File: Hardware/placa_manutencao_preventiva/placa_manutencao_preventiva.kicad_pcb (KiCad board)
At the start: 2 copper layers, 58.4 x 74.7 mm, 23 parts, among them J1 ENT_DIGITAL, J2 Power, J3 TESTE_TENSAO, J4 BAT_EXT, J5 BAT_HELTEC_CONN, J6 MPU6050, J7 BMP180, J8 Renewable energy, Q2 FQP30N06L, U1 Heltec_Wifi_LoRa_V1, U2 LM7805

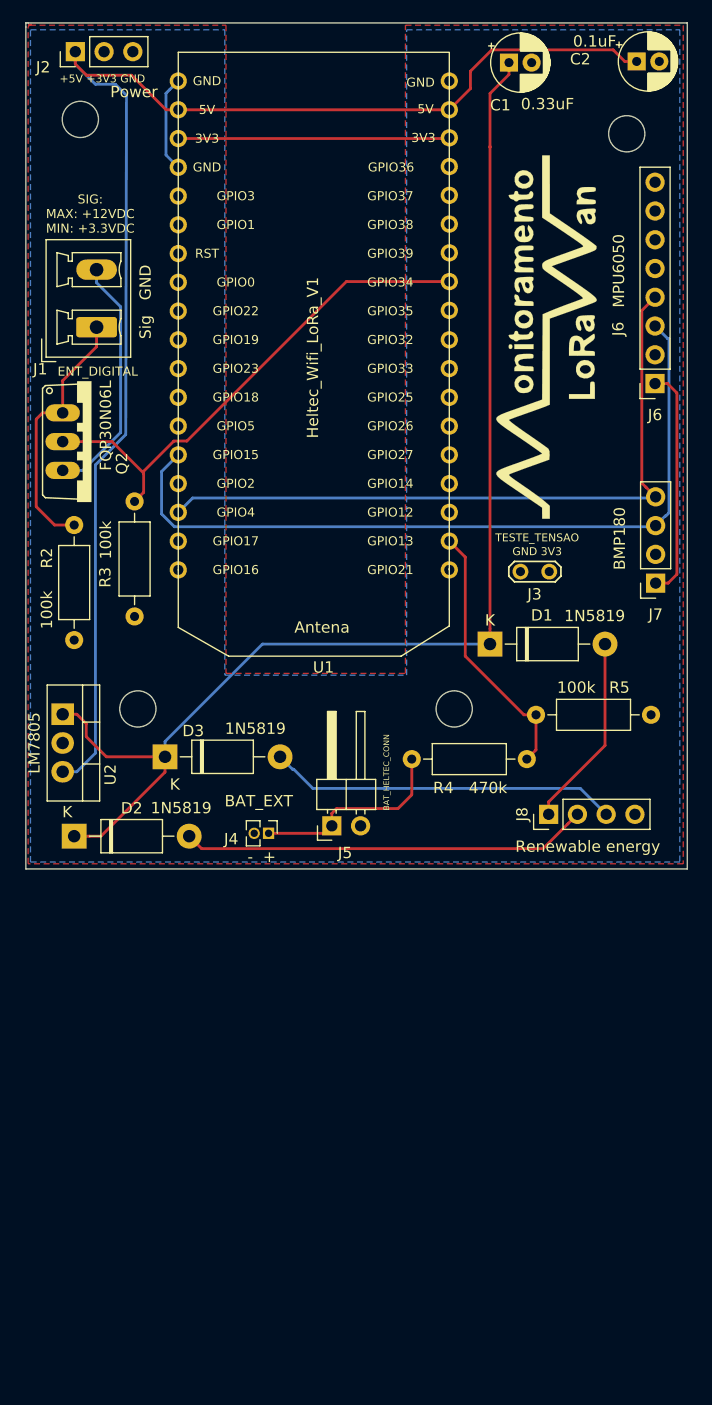
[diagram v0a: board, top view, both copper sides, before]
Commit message: Vers 1.1: Devolopment area
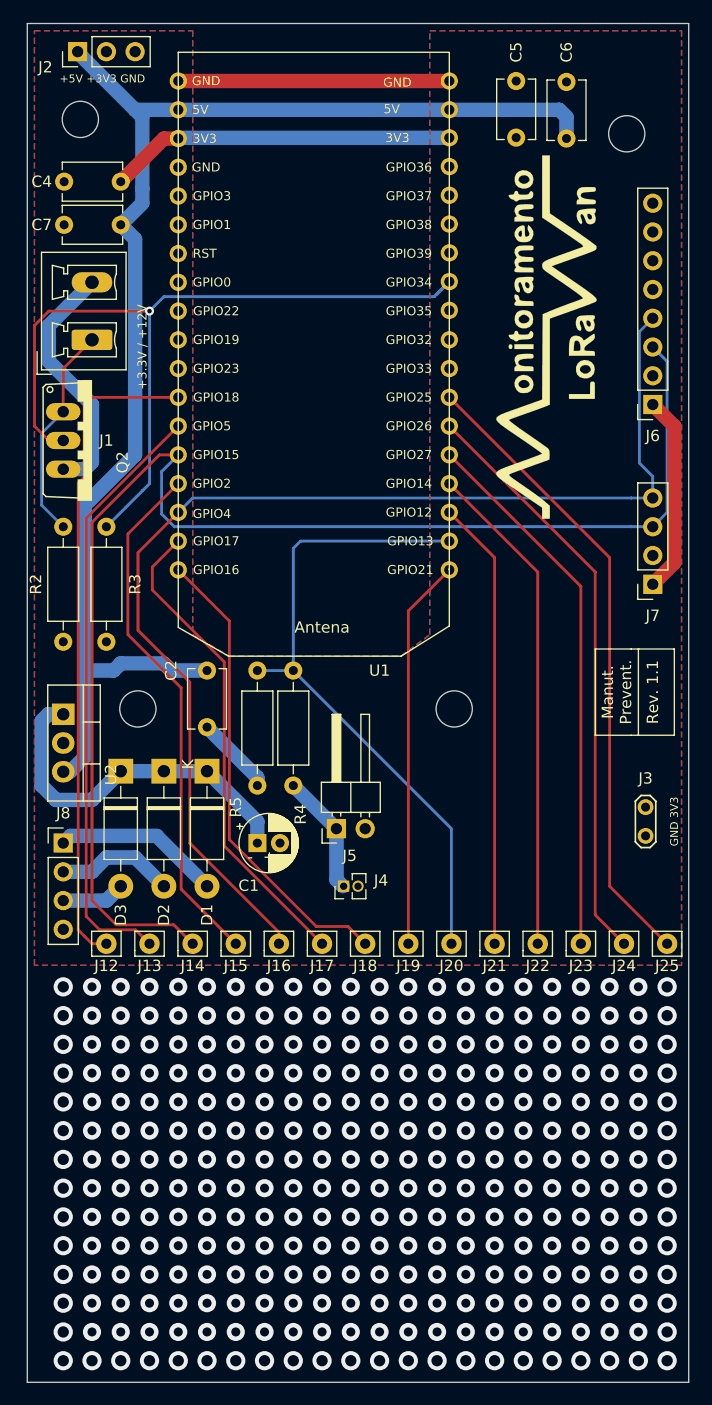
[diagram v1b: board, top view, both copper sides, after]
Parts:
- added C4: 0.1uF, Capacitor_THT:C_Disc_D5.1mm_W3.2mm_P5.00mm, F.Cu at (86.1, 29.0)
- added C5: 0.1uF, Capacitor_THT:C_Disc_D5.1mm_W3.2mm_P5.00mm, F.Cu at (121.0, 25.1)
- added C6: 0.1uF, Capacitor_THT:C_Disc_D5.1mm_W3.2mm_P5.00mm, F.Cu at (125.4, 25.1)
- added C7: 0.1uF, Capacitor_THT:C_Disc_D5.1mm_W3.2mm_P5.00mm, F.Cu at (86.1, 32.8)
- added J12: Conn_01x01, Connector_Pin:Pin_D0.9mm_L10.0mm_W2.4mm_FlatFork, F.Cu at (84.8, 96.3)
- added J13: Conn_01x01, Connector_Pin:Pin_D0.9mm_L10.0mm_W2.4mm_FlatFork, F.Cu at (88.6, 96.3)
- added J14: Conn_01x01, Connector_Pin:Pin_D0.9mm_L10.0mm_W2.4mm_FlatFork, F.Cu at (92.4, 96.3)
- added J15: Conn_01x01, Connector_Pin:Pin_D0.9mm_L10.0mm_W2.4mm_FlatFork, F.Cu at (96.2, 96.3)
- added J16: Conn_01x01, Connector_Pin:Pin_D0.9mm_L10.0mm_W2.4mm_FlatFork, F.Cu at (100.0, 96.3)
- added J17: Conn_01x01, Connector_Pin:Pin_D0.9mm_L10.0mm_W2.4mm_FlatFork, F.Cu at (103.8, 96.3)
- added J18: Conn_01x01, Connector_Pin:Pin_D0.9mm_L10.0mm_W2.4mm_FlatFork, F.Cu at (107.6, 96.3)
- added J19: Conn_01x01, Connector_Pin:Pin_D0.9mm_L10.0mm_W2.4mm_FlatFork, F.Cu at (111.5, 96.3)
- added J20: Conn_01x01, Connector_Pin:Pin_D0.9mm_L10.0mm_W2.4mm_FlatFork, F.Cu at (115.3, 96.3)
- added J21: Conn_01x01, Connector_Pin:Pin_D0.9mm_L10.0mm_W2.4mm_FlatFork, F.Cu at (119.1, 96.3)
- added J22: Conn_01x01, Connector_Pin:Pin_D0.9mm_L10.0mm_W2.4mm_FlatFork, F.Cu at (122.9, 96.3)
- added J23: Conn_01x01, Connector_Pin:Pin_D0.9mm_L10.0mm_W2.4mm_FlatFork, F.Cu at (126.7, 96.3)
- added J24: Conn_01x01, Connector_Pin:Pin_D0.9mm_L10.0mm_W2.4mm_FlatFork, F.Cu at (130.5, 96.3)
- added J25: Conn_01x01, Connector_Pin:Pin_D0.9mm_L10.0mm_W2.4mm_FlatFork, F.Cu at (134.3, 96.3)
- C1: value 0.33uF -> 10uF
- C2: footprint Capacitor_THT:CP_Radial_D5.0mm_P2.00mm -> Capacitor_THT:C_Disc_D5.1mm_W3.2mm_P5.00mm
- J4: value BAT_EXT -> BAT_EXT_JST_1.25mm
- U2: value LM7805 -> LM7805_TO220
- moved C1 72.4 mm to (98.1, 87.4)
- moved C2 65.8 mm to (93.7, 72.1), turned to 270 degrees
- moved J8 43.0 mm to (81.0, 87.4), turned to 0 degrees
- moved D1 27.4 mm to (93.7, 81.0), turned to 270 degrees
- moved R5 24.9 mm to (98.1, 72.1), turned to 270 degrees
- moved J3 22.5 mm to (132.4, 84.2), turned to 270 degrees
- moved R4 10.7 mm to (101.3, 82.3), turned to 90 degrees
- moved D2 9.79 mm to (89.9, 81.0), turned to 270 degrees
- moved J4 8.11 mm to (105.7, 91.2), turned to 90 degrees
- moved D3 4.11 mm to (86.1, 81.0), turned to 270 degrees
- moved R3 3.35 mm to (84.8, 69.6)
- moved J6 1.87 mm to (133.0, 48.6)
- moved J1 1.19 mm to (83.5, 42.9)
- moved R2 0.98 mm to (81.0, 59.4)
- moved J5 0.48 mm to (105.1, 86.1)
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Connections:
- J6 pad 5: (no net) -> Net-(J6-Pad5)
- J6 pad 6: (no net) -> Net-(J6-Pad6)
- J6 pad 7: (no net) -> Net-(J6-Pad7)
- J6 pad 8: (no net) -> Net-(J6-Pad8)
- U1 pad 10: (no net) -> Net-(U1-Pad10)
- U1 pad 11: (no net) -> Net-(U1-Pad11)
- U1 pad 12: (no net) -> Net-(J12-Pad1)
- U1 pad 13: (no net) -> Net-(J13-Pad1)
- U1 pad 15: (no net) -> Net-(J15-Pad1)
- U1 pad 17: (no net) -> Net-(J17-Pad1)
- U1 pad 18: (no net) -> Net-(J18-Pad1)
- U1 pad 19: (no net) -> Net-(J19-Pad1)
- U1 pad 21: (no net) -> Net-(J21-Pad1)
- U1 pad 22: (no net) -> Net-(J22-Pad1)
- U1 pad 23: (no net) -> Net-(J23-Pad1)
- U1 pad 24: (no net) -> Net-(J24-Pad1)
- U1 pad 25: (no net) -> Net-(J25-Pad1)
- U1 pad 26: (no net) -> Net-(U1-Pad26)
- U1 pad 27: (no net) -> Net-(U1-Pad27)
- U1 pad 28: (no net) -> Net-(U1-Pad28)
- U1 pad 30: (no net) -> Net-(U1-Pad30)
- U1 pad 31: (no net) -> Net-(U1-Pad31)
- U1 pad 32: (no net) -> Net-(U1-Pad32)
- U1 pad 33: (no net) -> Net-(U1-Pad33)
- U1 pad 5: (no net) -> Net-(U1-Pad5)
- U1 pad 6: (no net) -> Net-(U1-Pad6)
- U1 pad 7: (no net) -> Net-(U1-Pad7)
- U1 pad 8: (no net) -> Net-(U1-Pad8)
- U1 pad 9: (no net) -> Net-(U1-Pad9)
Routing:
- net Net-(C1-Pad1): track 108.8 -> 32.3 mm
- net Net-(J12-Pad1): track 0.00 -> 58.2 mm
- net Net-(J25-Pad1): track 0.00 -> 56.2 mm
- net Net-(J13-Pad1): track 0.00 -> 53.3 mm
- net Net-(J24-Pad1): track 0.00 -> 52.1 mm
- net I2C_SCL: track 68.7 -> 120.6 mm
- net Net-(J23-Pad1): track 0.00 -> 48.0 mm
- net Net-(J15-Pad1): track 0.00 -> 46.4 mm
- net Net-(J22-Pad1): track 0.00 -> 43.9 mm
- net I2C_SDA: track 61.4 -> 104.2 mm
- net Net-(J17-Pad1): track 0.00 -> 42.7 mm
- net Net-(J18-Pad1): track 0.00 -> 41.5 mm
- net Net-(J21-Pad1): track 0.00 -> 39.8 mm
- net ADC_BAT: track 23.4 -> 57.9 mm
- net Net-(J19-Pad1): track 0.00 -> 34.5 mm
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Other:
- board size 58.4 x 74.7 mm -> 58.4 x 120 mm
- net class Power added: clearance 0.2, trace_width 1.27, via_dia 0.8, via_drill 0.4
- board text added: "+3.3V / +12V"
- board text added: "Manut. Prevent."
- board text added: "Rev. 1.1"
- board text removed: "SIG: MAX: +12VDC MIN: +3.3VDC"
- board text removed: "Sig GND"
